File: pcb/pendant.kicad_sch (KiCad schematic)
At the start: 256 parts, among them J1 Conn_01x02, J2 USB_B_Micro, U1 ATSAMD21G18A-A, U2 LSM6DS3, U3 XC6206PxxxMR, U4 TP4057

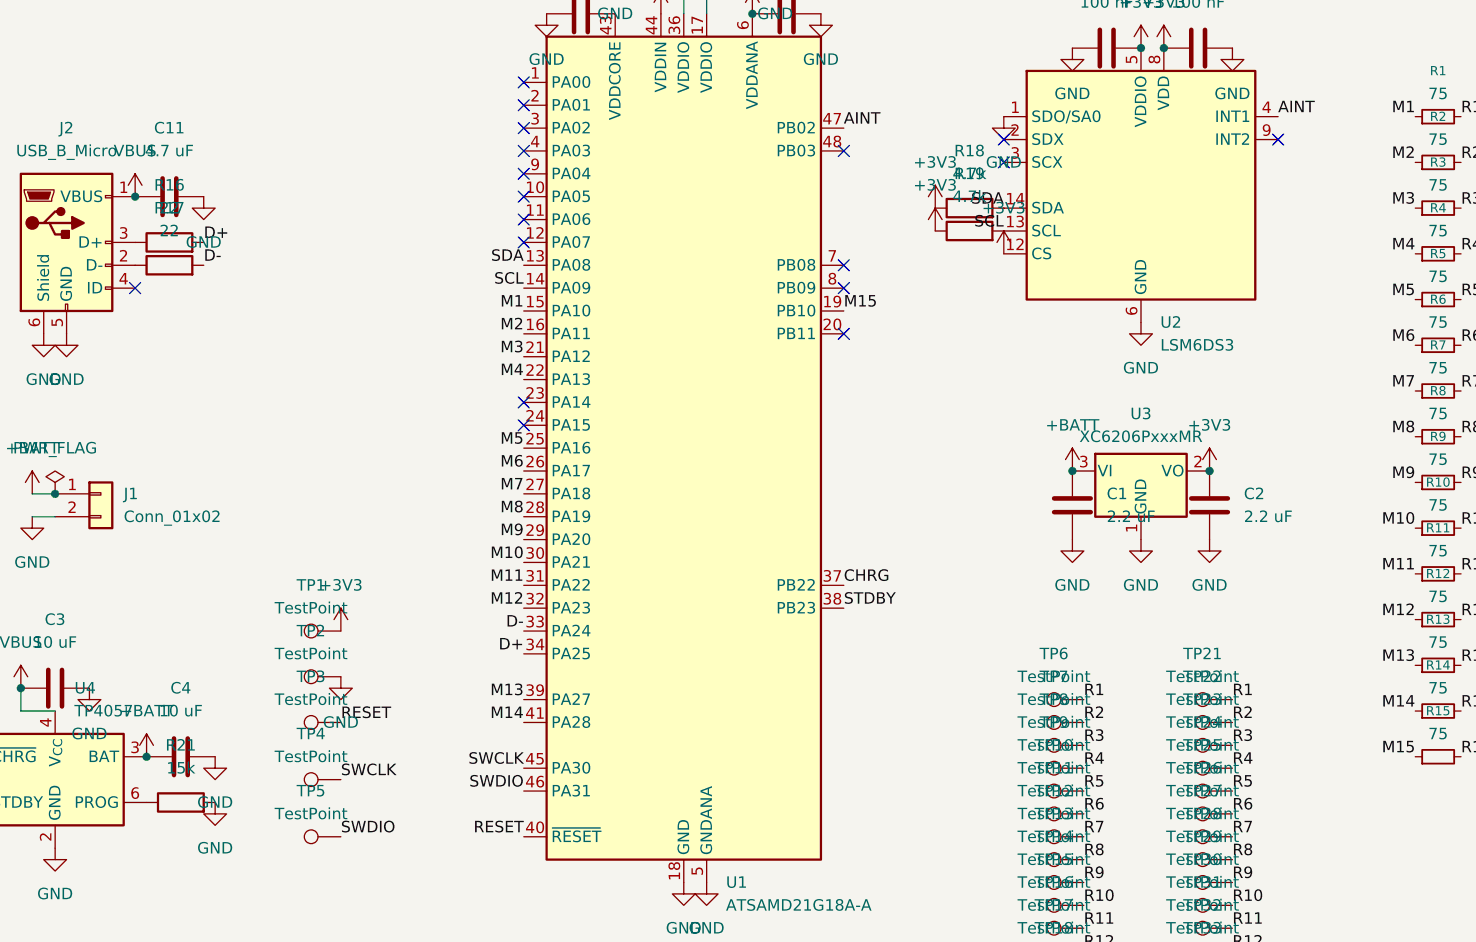
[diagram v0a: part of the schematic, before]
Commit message: Check values
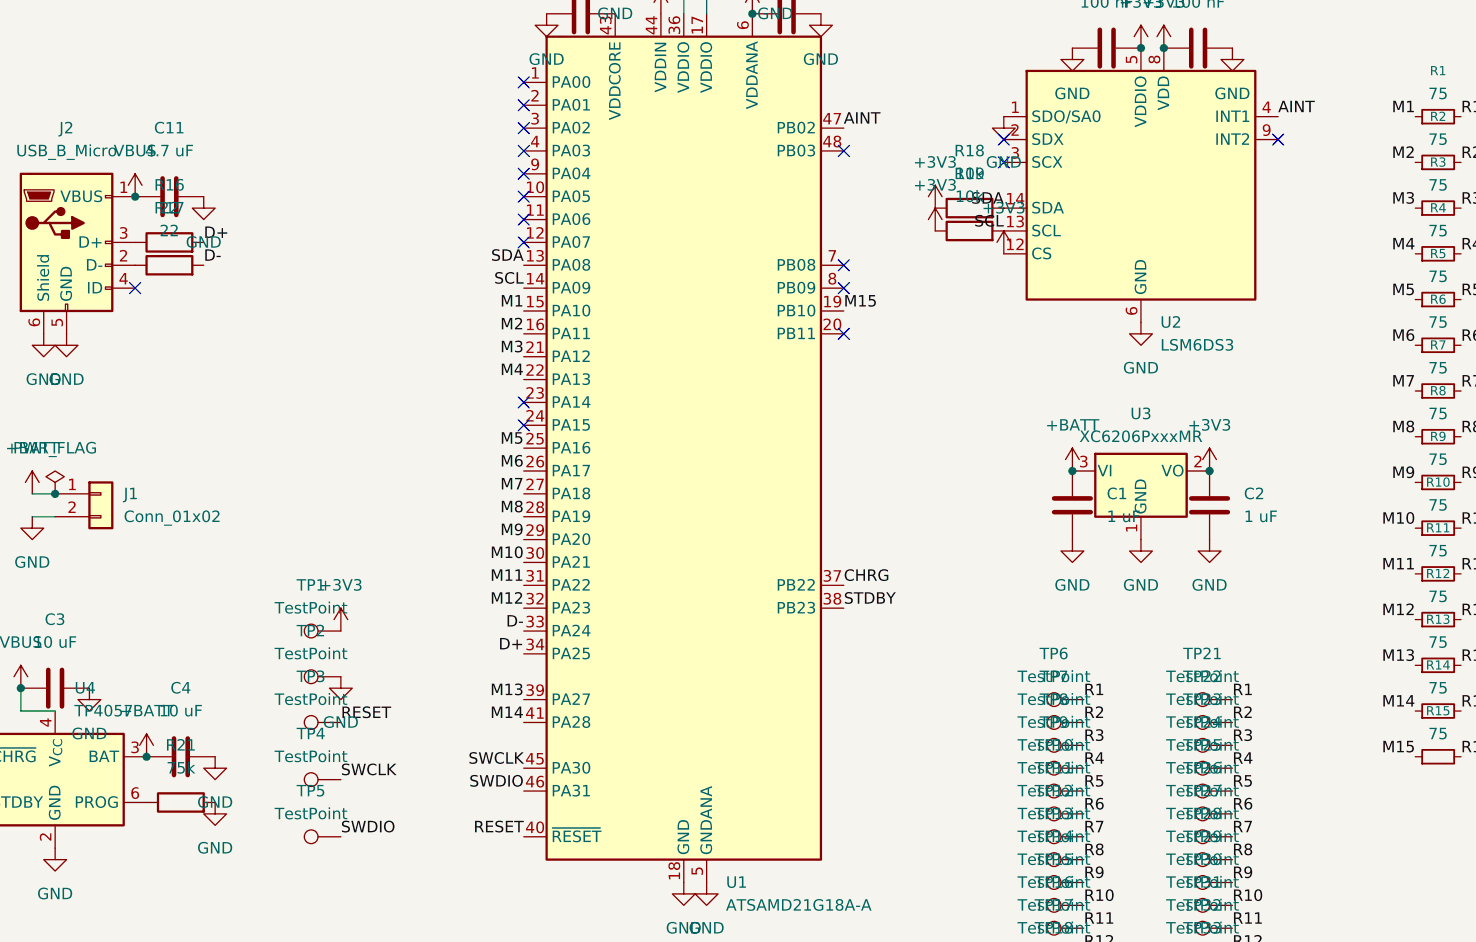
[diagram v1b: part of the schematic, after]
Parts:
- C1, C2: value 2.2 uF -> 1 uF
- R18, R19: value 4.7k -> 10k
- R21: value 15k -> 75k
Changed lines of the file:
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@@
 			)
 		)
-		(property "Value" "4.7k"
+		(property "Value" "10k"
 			(at 139.7 57.15 90)
 			(show_name no)
@@
 			)
 		)
-		(property "Value" "4.7k"
+		(property "Value" "10k"
 			(at 139.7 54.61 90)
 			(show_name no)
@@
 			)
 		)
-		(property "Value" "2.2 uF"
+		(property "Value" "1 uF"
 			(at 170.18 92.7099 0)
 			(show_name no)
@@
 			)
 		)
-		(property "Value" "2.2 uF"
+		(property "Value" "1 uF"
 			(at 154.94 92.7099 0)
 			(show_name no)
@@
 			)
 		)
-		(property "Value" "15k"
+		(property "Value" "75k"
 			(at 52.07 120.65 90)
 			(show_name no)
